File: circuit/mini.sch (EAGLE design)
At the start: 82 parts, among them IC1 74AC4053D, IC2 74AC74D, IC3 STM32L151CBT6, IC4 MCP1700-3.3V, IC5 NE5534D, IC6 NE5534D, Q1 BFG135, Q2 8MHz, X1 1-227161-0, X4 MINI-USB

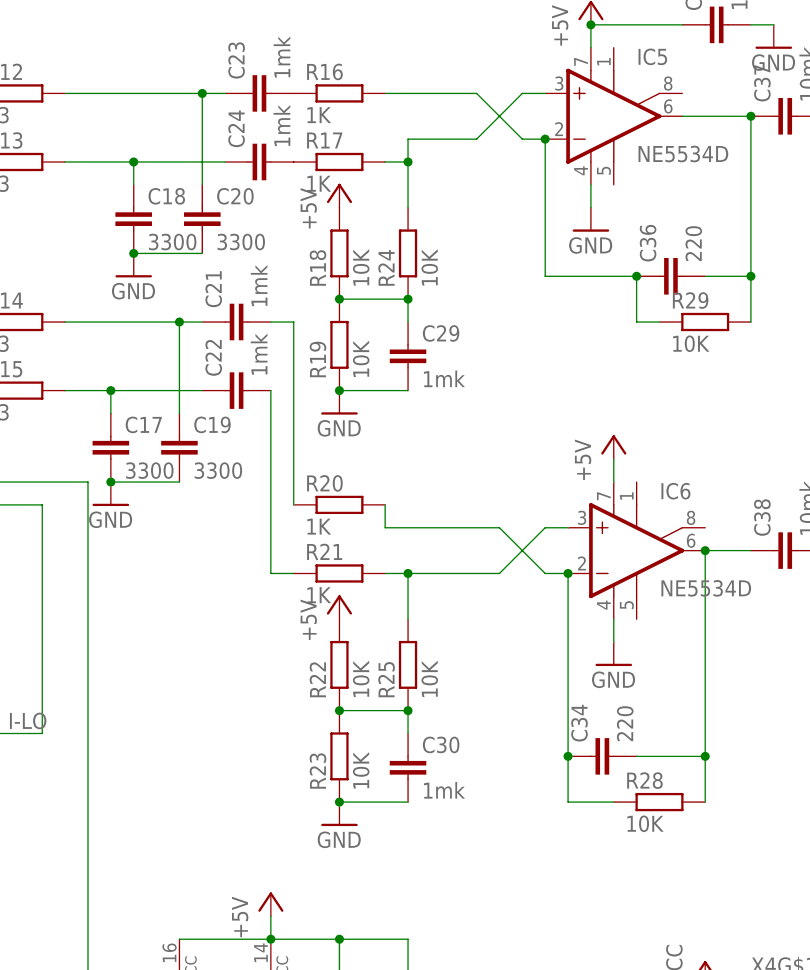
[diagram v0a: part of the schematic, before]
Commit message: - ?????? ???? ?????? ??????? ????? ??
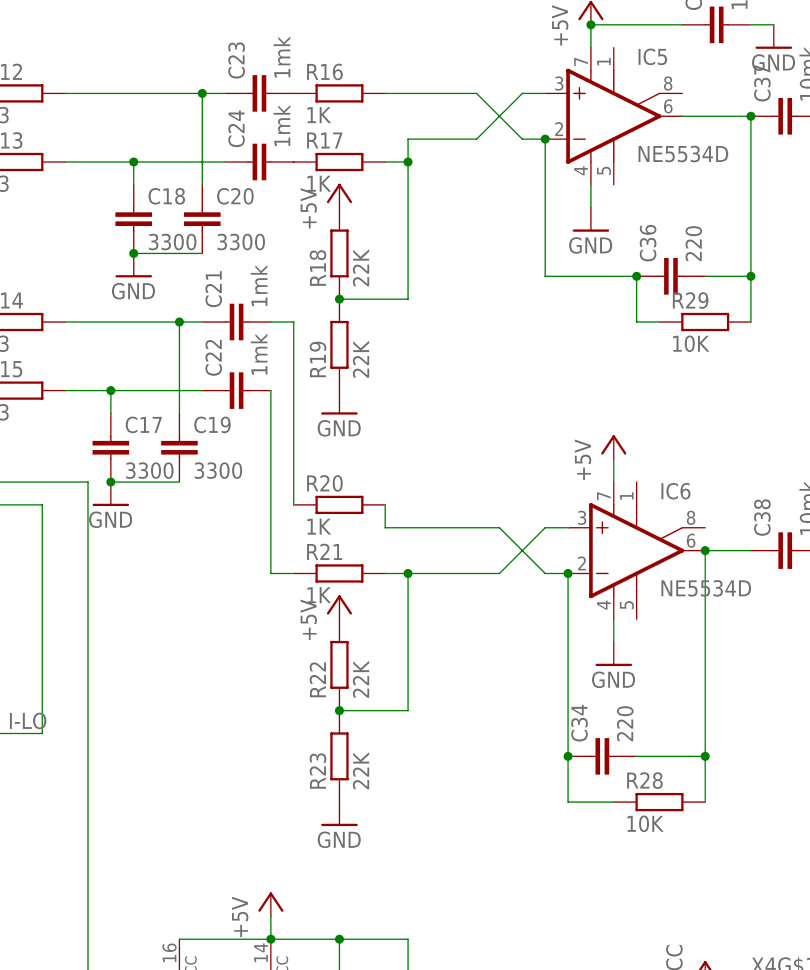
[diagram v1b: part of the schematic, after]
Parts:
- removed C29, C30: 1mk, rcl:C-EUC0603
- removed R24, R25: 10K, rcl:R-EU_R0603
- R18, R19, R22, R23: value 10K -> 22K
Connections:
- removed net N$24: IC6.+IN, R21.2, R25.2
- removed net N$26: IC5.+IN, R17.2, R24.2
- net GND: no longer C29.2, C30.2
- net N$15: now also IC5.+IN, R17.2; no longer C29.1, R24.1
- net N$23: now also IC6.+IN, R21.2; no longer C30.1, R25.1
